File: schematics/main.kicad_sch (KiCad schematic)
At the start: 2 parts

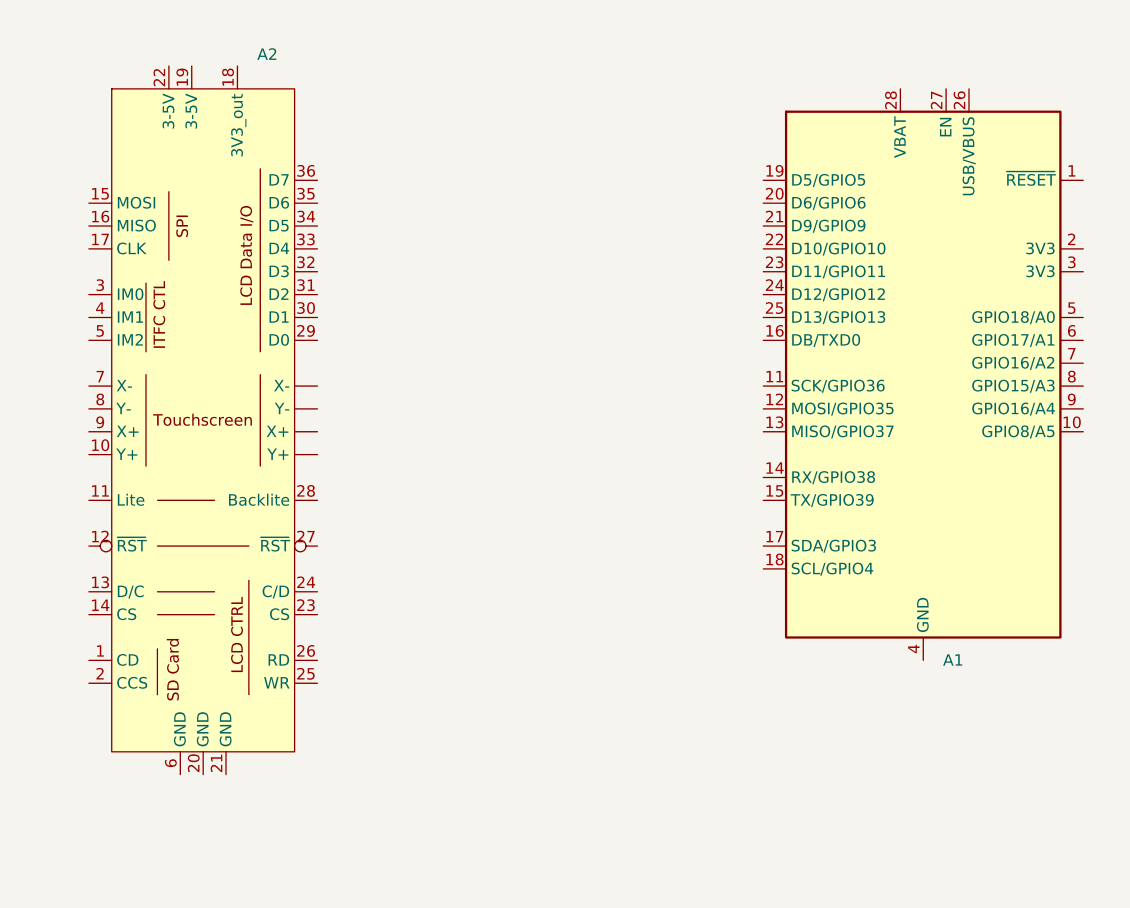
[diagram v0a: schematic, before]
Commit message: Finish schematics
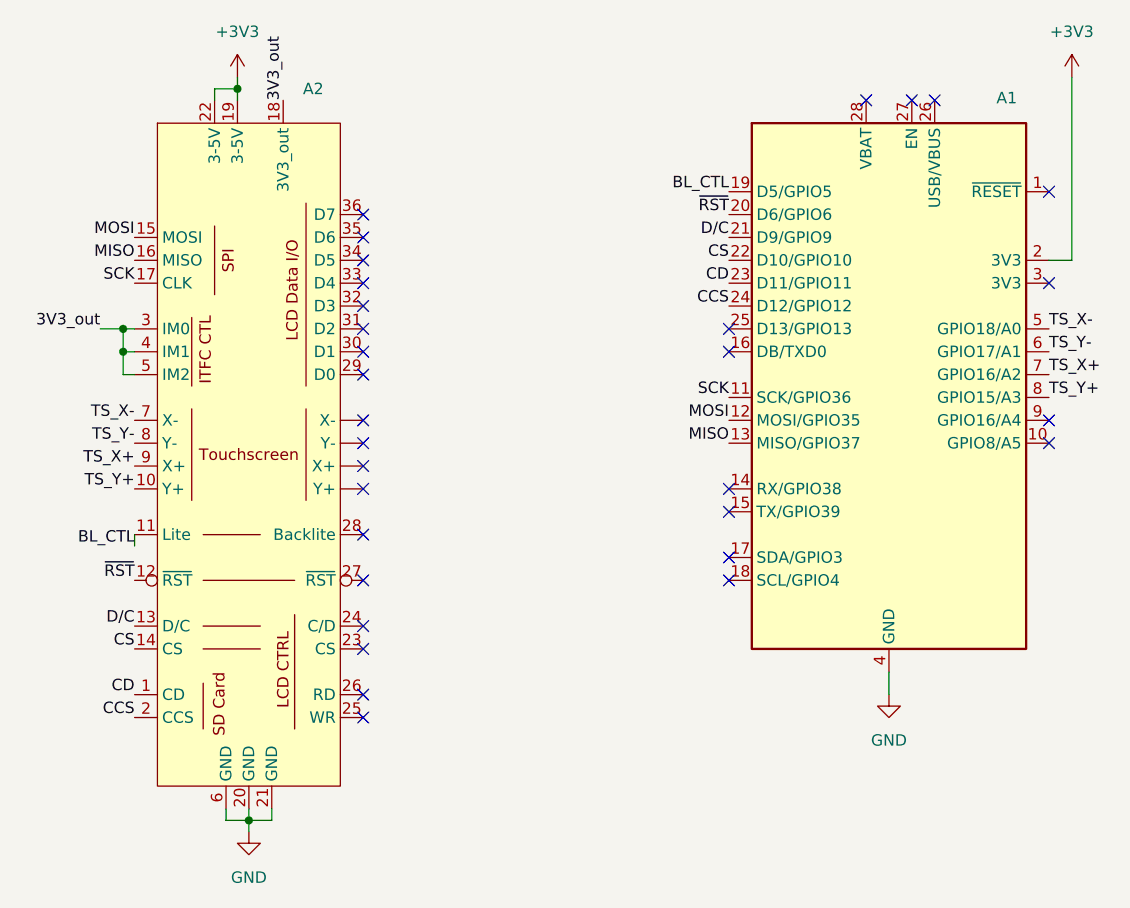
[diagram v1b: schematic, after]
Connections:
- net SCK: now reaches A1.11 (SCK/GPIO36)
- net SCK: now also A2.17 (CLK)
- net MOSI: now reaches A1.12 (MOSI/GPIO35)
- net MOSI: now also A2.15 (MOSI)
- net MISO: now reaches A1.13 (MISO/GPIO37)
- net MISO: now also A2.16 (MISO)
- net BL_CTL: now reaches A1.19 (D5/GPIO5)
- net BL_CTL: now also A2.11 (Lite)
- net +3V3: now reaches A1.2 (3V3)
- net +3V3: now also A2.19 (3-5V), A2.22 (3-5V)
- net ~{RST}: now reaches A1.20 (D6/GPIO6)
- net ~{RST}: now also A2.12 (~{RST})
- net D/C: now reaches A1.21 (D9/GPIO9)
- net D/C: now also A2.13 (D/C)
- net CS: now reaches A1.22 (D10/GPIO10)
- net CS: now also A2.14 (CS)
- net CD: now reaches A1.23 (D11/GPIO11)
- net CD: now also A2.1 (CD)
- net CCS: now reaches A1.24 (D12/GPIO12)
- net CCS: now also A2.2 (CCS)
- net GND: now reaches A1.4 (GND)
- net GND: now also A2.20 (GND), A2.21 (GND), A2.6 (GND)
- net TS_X-: now reaches A1.5 (GPIO18/A0)
- net TS_X-: now also A2.7 (X-)
- net TS_Y-: now reaches A1.6 (GPIO17/A1)
- net TS_Y-: now also A2.8 (Y-)
- net TS_X+: now reaches A1.7 (GPIO16/A2)
- net TS_X+: now also A2.9 (X+)
- net TS_Y+: now reaches A1.8 (GPIO15/A3)
- net TS_Y+: now also A2.10 (Y+)
- net 3V3_out: now reaches A2.18 (3V3_out)
- net 3V3_out: now also A2.3 (IM0), A2.4 (IM1), A2.5 (IM2)
- no-connect marks 0 -> 31
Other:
- moved on the sheet: A1, A2
